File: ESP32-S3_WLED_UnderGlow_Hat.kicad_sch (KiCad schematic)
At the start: 0 parts

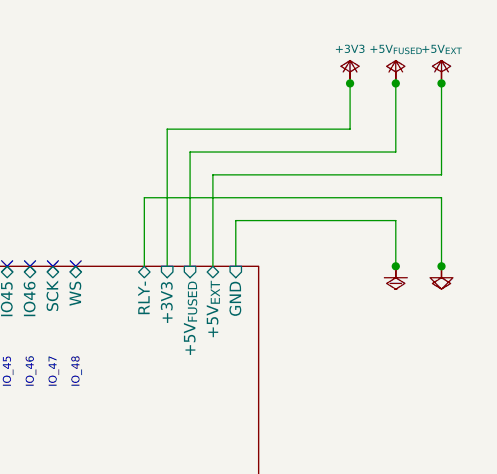
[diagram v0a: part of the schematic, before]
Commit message: Update .gitignore, CANBus_Interface.kicad_sch, ESP32-S3_WLED_UnderGlow_Hat-2026-05-04_233126.zip, and 17 more files
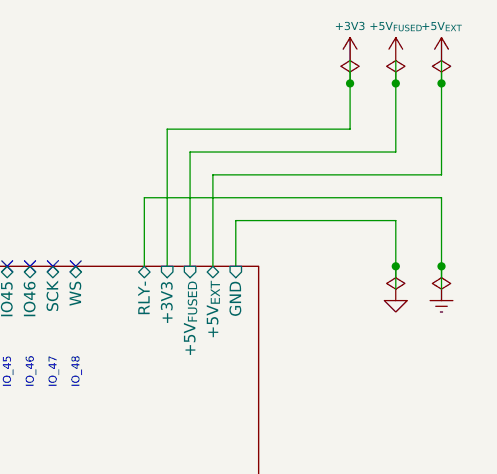
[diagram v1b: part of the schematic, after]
